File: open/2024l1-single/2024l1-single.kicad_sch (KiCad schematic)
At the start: 89 parts, among them IC1 LM2587S-ADJ, J1 Conn_01x03, J2 Conn_01x03, J3 Conn_01x02, J4 Conn_01x02, J6 Conn_01x04, U1 Seeed Studio XIAO SAMD21, U2 CD74HC4067SM

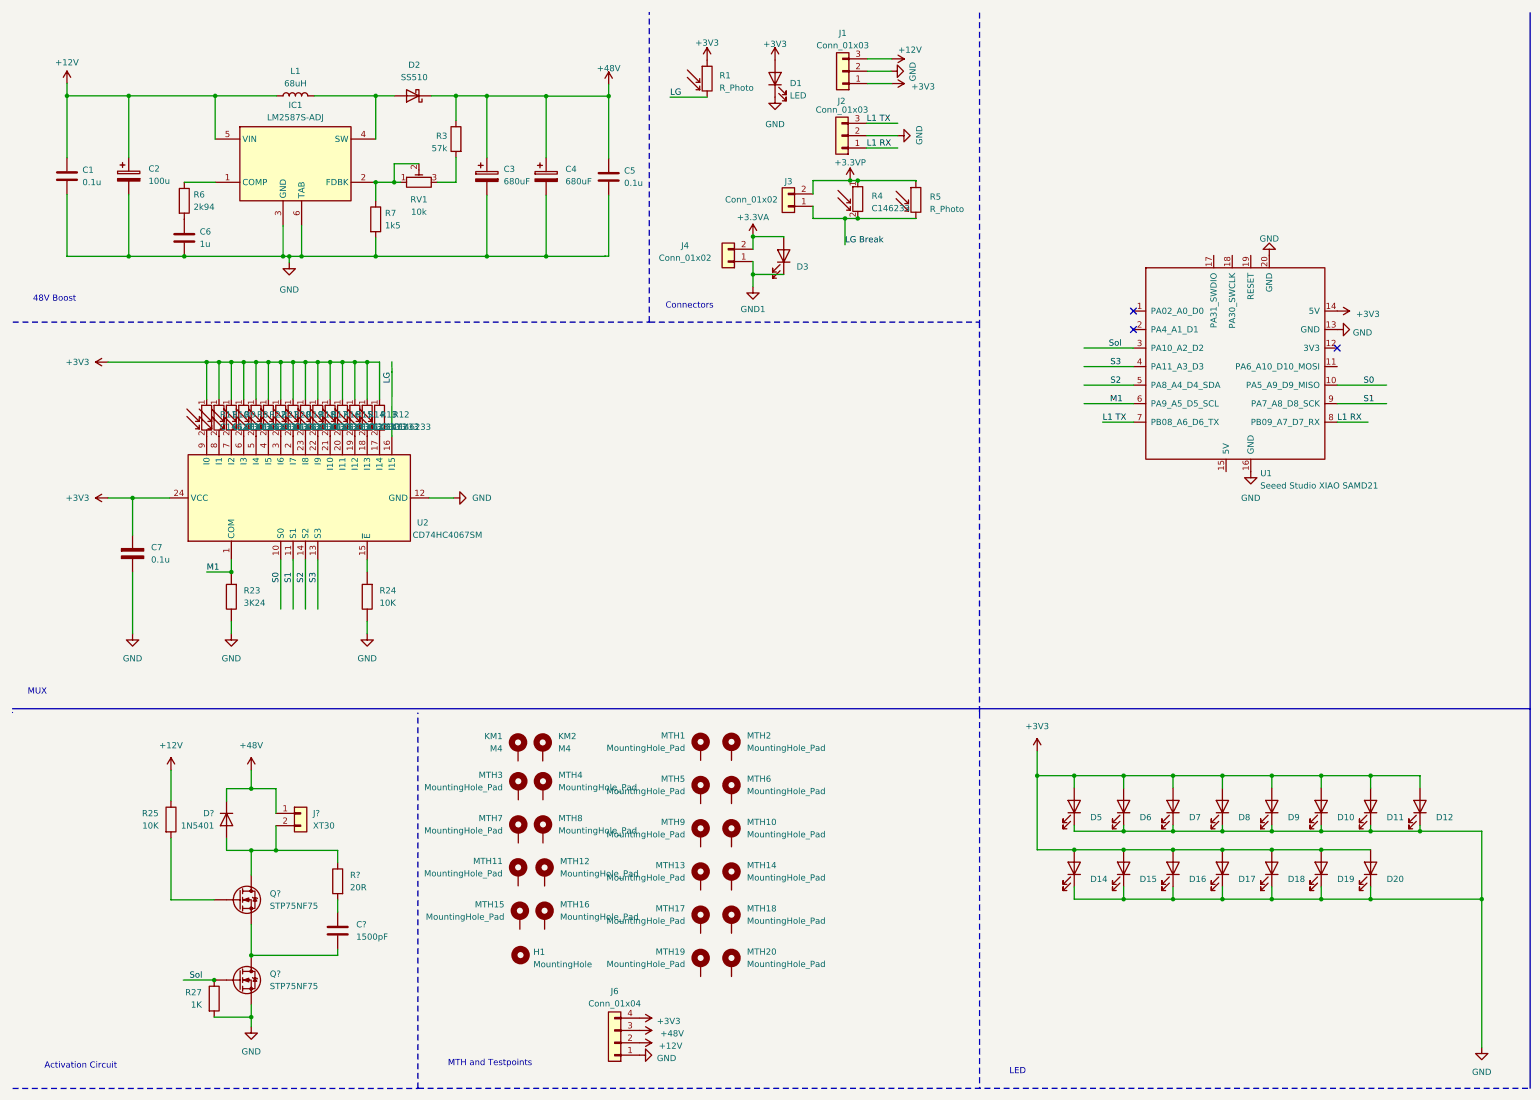
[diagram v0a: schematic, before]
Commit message: reformatted
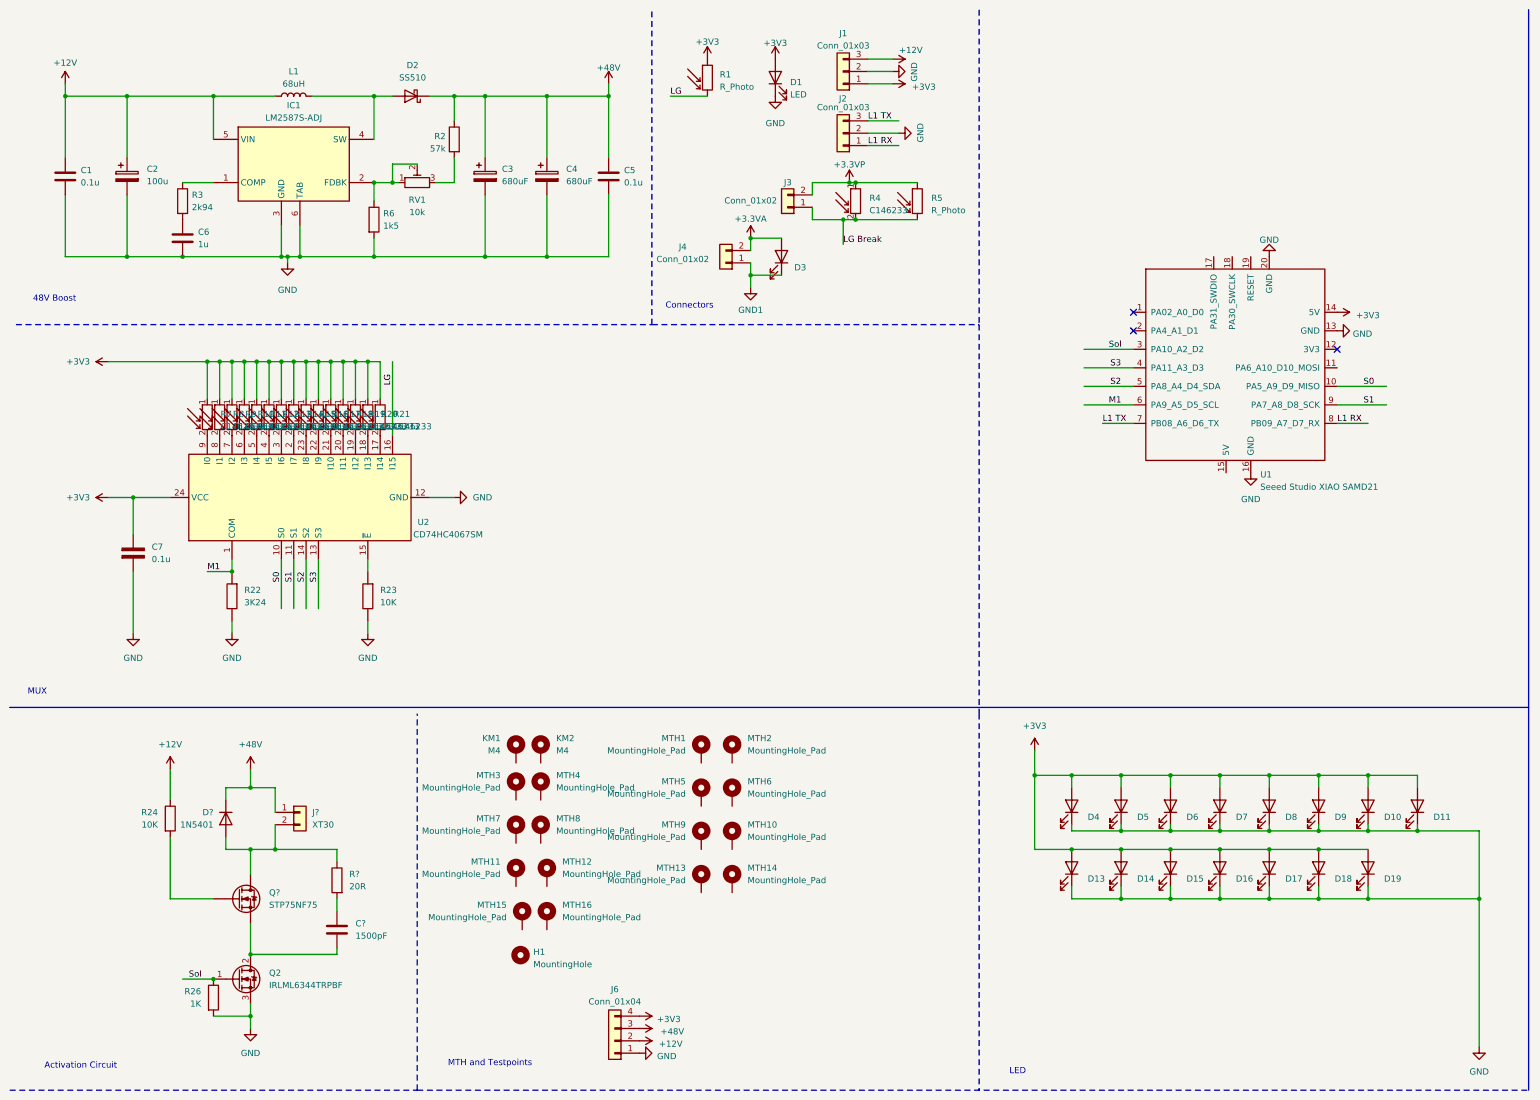
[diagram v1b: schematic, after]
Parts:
- removed MTH17, MTH18, MTH19, MTH20: MountingHole_Pad, MountingHole:MountingHole_3.2mm_M3_Pad_Via, symbol Mechanical:MountingHole_Pad
- removed Q?: STP75NF75, 2024l1:TO255P1040X460X2890-3, symbol vincent:IPD050N10N5ATMA1
- added Q2: IRLML6344TRPBF, SOT95P237X112-3N, symbol vincent:IRLML6344TRPBF
- renumbered D11 to D10, D12 to D11, D14 to D13, D15 to D14, D16 to D15, D17 to D16, D18 to D17, D19 to D18, D20 to D19, D5 to D4, D6 to D5, D7 to D6, D8 to D7, D9 to D8, D10 to D9, R8 to R10, R22 to R11, R21 to R12, R20 to R13, R19 to R14, R18 to R15, R17 to R16, R16 to R17, R15 to R18, R14 to R19, R3 to R2, R13 to R20, R12 to R21, R23 to R22, R24 to R23, R25 to R24, R27 to R26, R6 to R3, R7 to R6, R11 to R7, R10 to R8
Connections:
- net GND: now also Q2.3 (S)
- net Sol: now also Q2.1 (G)
- net at C?.2, Q?.3 (S): now also Q2.2 (D)
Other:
- moved on the sheet: D10, D11, D13, D14, D15, D16, D17, D18, D19, D4, D5, D6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

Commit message: Restored L1 Footprint Library
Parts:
- C1, C5, C6, C7, C?: footprint 2024l1:cap0603 -> 2024l1 Single:cap0603
- D10, D11, D13, D14, D15, D16, D17, D18, D19, D3, D4, D5, D6, D7, D8, D9: footprint 2024l1:C2843867 -> 2024l1 Single:C2843867
- D2: footprint 2024l1:SMA (DO-214AC) -> 2024l1 Single:SMA (DO-214AC)
- H1: footprint 2024l1:SEN Logo Mini -> 2024l1 Single:SEN Logo Mini
- IC1: footprint 2024l1:TO170P1435X465-6N -> 2024l1 Single:TO170P1435X465-6N
- J6: footprint 2024l1:14 AWG 4 Holes -> 2024l1 Single:14 AWG 4 Holes
- J?: footprint 2024l1:AMASS_XT30-F -> 2024l1 Single:AMASS_XT30-F
- L1: footprint 2024l1:1040 One Piece Inductor -> 2024l1 Single:1040 One Piece Inductor
- Q2: footprint SOT95P237X112-3N -> 2024l1 Single:SOT95P237X112-3N
- Q?: footprint 2024l1:TO255P1040X460X2890-3 -> 2024l1 Single:TO255P1040X460X2890-3
- R10, R11, R12, R13, R14, R15, R16, R17, R18, R19, R20, R21, R4, R7, R8, R9: footprint 2024l1:C146233 -> 2024l1 Single:C146233
- R2, R22, R23, R24, R26, R3, R6, R?: footprint 2024l1:res0603 -> 2024l1 Single:res0603
- R5: footprint 2024l1:Through Hole LDR -> 2024l1 Single:Through Hole LDR
- RV1: footprint 2024l1:TRIM_3362W-1-203LF -> 2024l1 Single:TRIM_3362W-1-203LF
- U1: footprint 2024l1:Seeeduino XIAO SAMD 21 TFT -> 2024l1 Single:Seeeduino XIAO SAMD 21 TFT
- U2: footprint 2024l1:CD74HC4067M -> 2024l1 Single:CD74HC4067M

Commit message: L3 - SCH
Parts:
- C2: footprint Capacitor_SMD:CP_Elec_10x10.5 -> Capacitor_SMD:CP_Elec_8x10.5
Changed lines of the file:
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@@
       (effects (font (size 1.27 1.27)) (justify left))
     )
-    (property "Footprint" "Capacitor_SMD:CP_Elec_10x10.5" (at 36.5252 49.53 0)
+    (property "Footprint" "Capacitor_SMD:CP_Elec_8x10.5" (at 36.5252 49.53 0)
       (effects (font (size 1.27 1.27)) hide)
     )
